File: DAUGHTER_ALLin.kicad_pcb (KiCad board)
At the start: 2 copper layers, 43.5 x 27 mm, 15 parts, among them IC1 SN6501-Q1, J1 Conn_02x08_Odd_Even, T1 760390012, U1 IZL10T1A-SOIC8

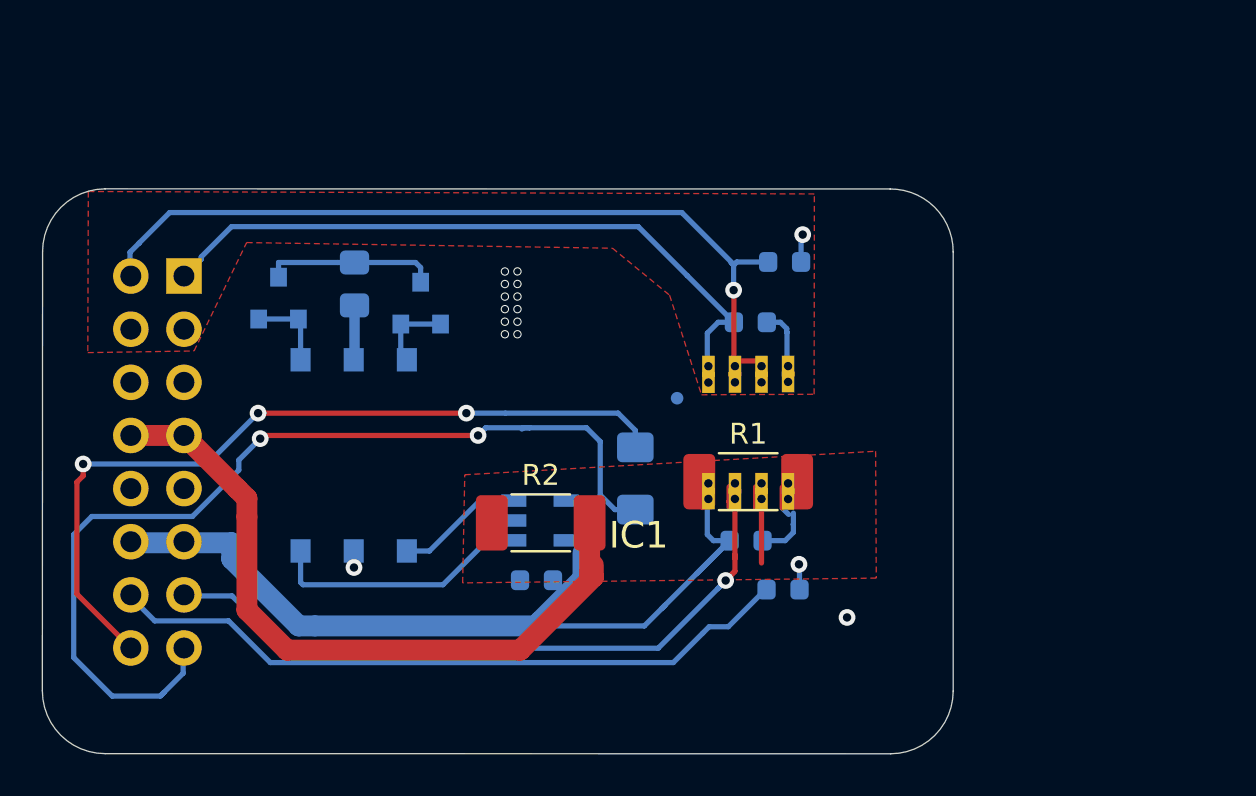
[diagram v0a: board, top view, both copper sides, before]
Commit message: multicb version
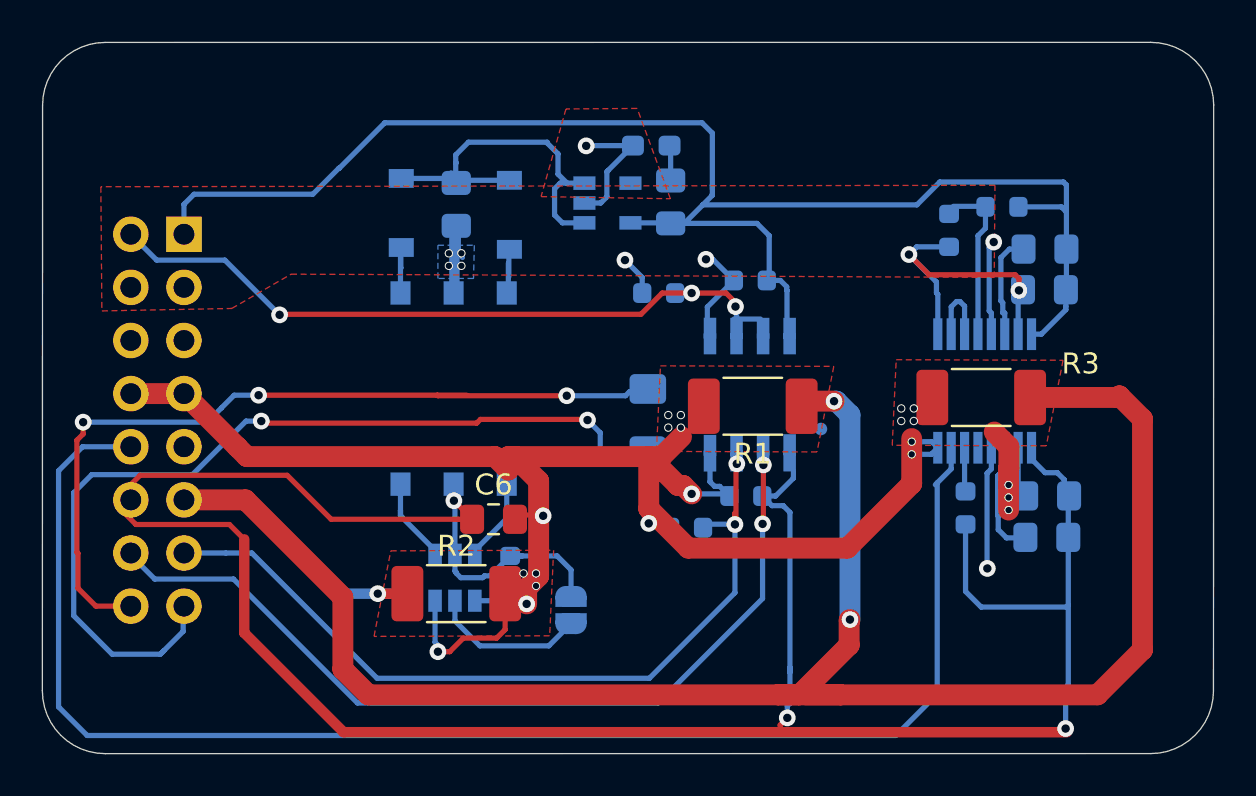
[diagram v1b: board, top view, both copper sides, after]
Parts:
- added C10: C_0805_1u, Capacitor_SMD:C_0805_2012Metric_Pad1.15x1.40mm_HandSolder, B.Cu at (120.8, 100.7)
- added C11: C_0805, Capacitor_SMD:C_0805_2012Metric_Pad1.15x1.40mm_HandSolder, B.Cu at (102.9, 96.5)
- added C6: C_0805, Capacitor_SMD:C_0805_2012Metric_Pad1.15x1.40mm_HandSolder, F.Cu at (94.5, 111.7)
- added C7: C_0805_1u, Capacitor_SMD:C_0805_2012Metric_Pad1.15x1.40mm_HandSolder, B.Cu at (121.0, 110.6)
- added C8: C_0805_1u, Capacitor_SMD:C_0805_2012Metric_Pad1.15x1.40mm_HandSolder, B.Cu at (120.9, 112.5)
- added C9: C_0805_1u, Capacitor_SMD:C_0805_2012Metric_Pad1.15x1.40mm_HandSolder, B.Cu at (120.8, 98.8)
- added JP1: SolderJumper_2_Open_VDDTECH, Jumper:SolderJumper-2_P1.3mm_Open_RoundedPad1.0x1.5mm, B.Cu at (98.2, 116.0)
- added R3: Heater, Resistor_SMD:R_2010_5025Metric_Pad1.52x2.65mm_HandSolder, F.Cu at (117.8, 105.9)
- added R4: 10k R_0603, Resistor_SMD:R_0603_1608Metric, B.Cu at (117.0, 111.1)
- added R7: 10k R_0603, Resistor_SMD:R_0603_1608Metric, B.Cu at (118.8, 96.7)
- added R8: 10k R_0603, Resistor_SMD:R_0603_1608Metric, B.Cu at (116.2, 97.9)
- added R9: R_0603, Resistor_SMD:R_0603_1608Metric_Pad1.05x0.95mm_HandSolder, B.Cu at (102.0, 93.8)
- added U2: SN6505BDBV, Package_TO_SOT_SMD:SOT-23-6, B.Cu at (92.6, 114.5)
- added U3: TPS76350, Package_TO_SOT_SMD:SOT-23-5, B.Cu at (99.9, 96.6)
- D1, D2: value BAT54C_SOT23 -> MBR0520; footprint Package_TO_SOT_SMD:SOT-23 -> Diode_SMD:D_SOD-123
- IC1: value SN6501-Q1 -> ADUM3190BRQZ; footprint VDDTECH_FOOTPRINTS:SOT95P280X145-5N -> VDDTECH_FOOTPRINTS:SOP64P600X175-16N
- U1: footprint VDDTECH_FOOTPRINTS:SOIC8_typ_HEAT -> VDDTECH_FOOTPRINTS:SOIC8_typ_HEAT_no_vias
- moved IC1 22.1 mm to (117.9, 105.5), turned to 90 degrees
- moved D2 7.14 mm to (90.1, 97.0), turned to 270 degrees
- moved R6 6.20 mm to (102.4, 100.9), turned to 0 degrees
- moved C5 6.17 mm to (92.7, 96.6)
- moved D1 5.99 mm to (95.2, 97.1), turned to 270 degrees
- moved T1 5.74 mm to (92.6, 105.4)
- moved C1 5.48 mm to (103.7, 112.1), turned to 180 degrees
- moved R2 5.27 mm to (92.7, 115.2)
- moved R1 3.61 mm to (106.9, 106.3), turned to 180 degrees
- moved R5 2.86 mm to (101.8, 106.9)
- moved U1 2.71 mm to (106.7, 108.0), turned to 90 degrees
- moved C2 2.13 mm to (106.5, 110.6), turned to 180 degrees
- moved C3 2.00 mm to (106.7, 100.3), turned to 180 degrees
- moved J1 2.00 mm to (79.7, 98.1)
- moved C4 1.31 mm to (95.3, 114.2), turned to 270 degrees
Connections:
- C5 pad 1: /VDDH -> Net-(C5-Pad1)
- C5 pad 2: Net-(C5-Pad2) -> /VSH
- D1 pad 1: Net-(D1-Pad1) -> Net-(C5-Pad1)
- D1 pad 2: Net-(D1-Pad1) -> Net-(D1-Pad2)
- D2 pad 1: Net-(D2-Pad1) -> Net-(C5-Pad1)
- D2 pad 2: Net-(D2-Pad1) -> Net-(D2-Pad2)
- IC1 pad 1: Net-(IC1-Pad1) -> /VDD
- IC1 pad 2: /VDD -> GND
- IC1 pad 3: Net-(IC1-Pad3) -> /VREG1
- IC1 pad 4: GND -> /REFOUT1
- IC1 pad 5: GND -> Net-(IC1-Pad5)
- J1 pad 10: /R_HEAT_SW -> /EAOUT
- J1 pad 11: /VDD -> /VDD_heat
- J1 pad 13: /INH_OUT -> /INH_buf
- J1 pad 14: /INH_buf -> /INH_OUT
- J1 pad 9: /R_HEAT_SW -> Net-(J1-Pad9)
- R1 pad 1: /VDD -> /VDD_heat
- R2 pad 1: /VDD -> /VDD_heat
- T1 pad 1: Net-(IC1-Pad3) -> Net-(T1-Pad1)
- T1 pad 3: Net-(IC1-Pad1) -> Net-(T1-Pad3)
- T1 pad 4: Net-(D2-Pad1) -> Net-(D2-Pad2)
- T1 pad 5: Net-(C5-Pad2) -> /VSH
- T1 pad 6: Net-(D1-Pad1) -> Net-(D1-Pad2)
- U1 pad 1: /VDDH -> /VDD
- U1 pad 2: /INH_ISO -> /INH_OUT
- U1 pad 3: /INH_ISO -> /INH_buf
- U1 pad 4: /VSH -> GND
- U1 pad 5: GND -> /VSH
- U1 pad 6: /INH_buf -> /INH_ISO
- U1 pad 7: /INH_OUT -> /INH_ISO
- U1 pad 8: /VDD -> /VDDH
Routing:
- net /VDD_heat: track 0.00 -> 102.9 mm, vias 0 -> 3
- net /VDD: track 43.6 -> 123.1 mm, vias 1 -> 3
- net /EAOUT: track 0.00 -> 70.8 mm
- net GND: track 39.4 -> 89.0 mm, vias 1 -> 21
- net /VDDH: track 41.4 -> 75.4 mm, vias 1 -> 0
- net /VSH: track 5.00 -> 33.9 mm, vias 1 -> 9
- net Net-(C5-Pad1): track 0.00 -> 17.8 mm
- net Net-(IC1-Pad1): track 12.6 -> 0.00 mm
- net Net-(IC1-Pad12): track 0.00 -> 7.78 mm
- net Net-(JP1-Pad2): track 0.00 -> 7.45 mm
- net /INH_OUT: track 34.9 -> 42.2 mm, vias 1 -> 2
- net Net-(IC1-Pad3): track 6.11 -> 0.00 mm
- net /INH_ISO: track 41.7 -> 35.9 mm, vias 1 -> 3
- net /REFOUT1: track 0.00 -> 5.86 mm, vias 0 -> 1
- net /VREG1: track 0.00 -> 5.74 mm
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- added copper zone on B.Cu, net /VSH
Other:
- board size 43.5 x 27 mm -> 56 x 34 mm
